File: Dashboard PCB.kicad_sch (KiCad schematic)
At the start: 40 parts

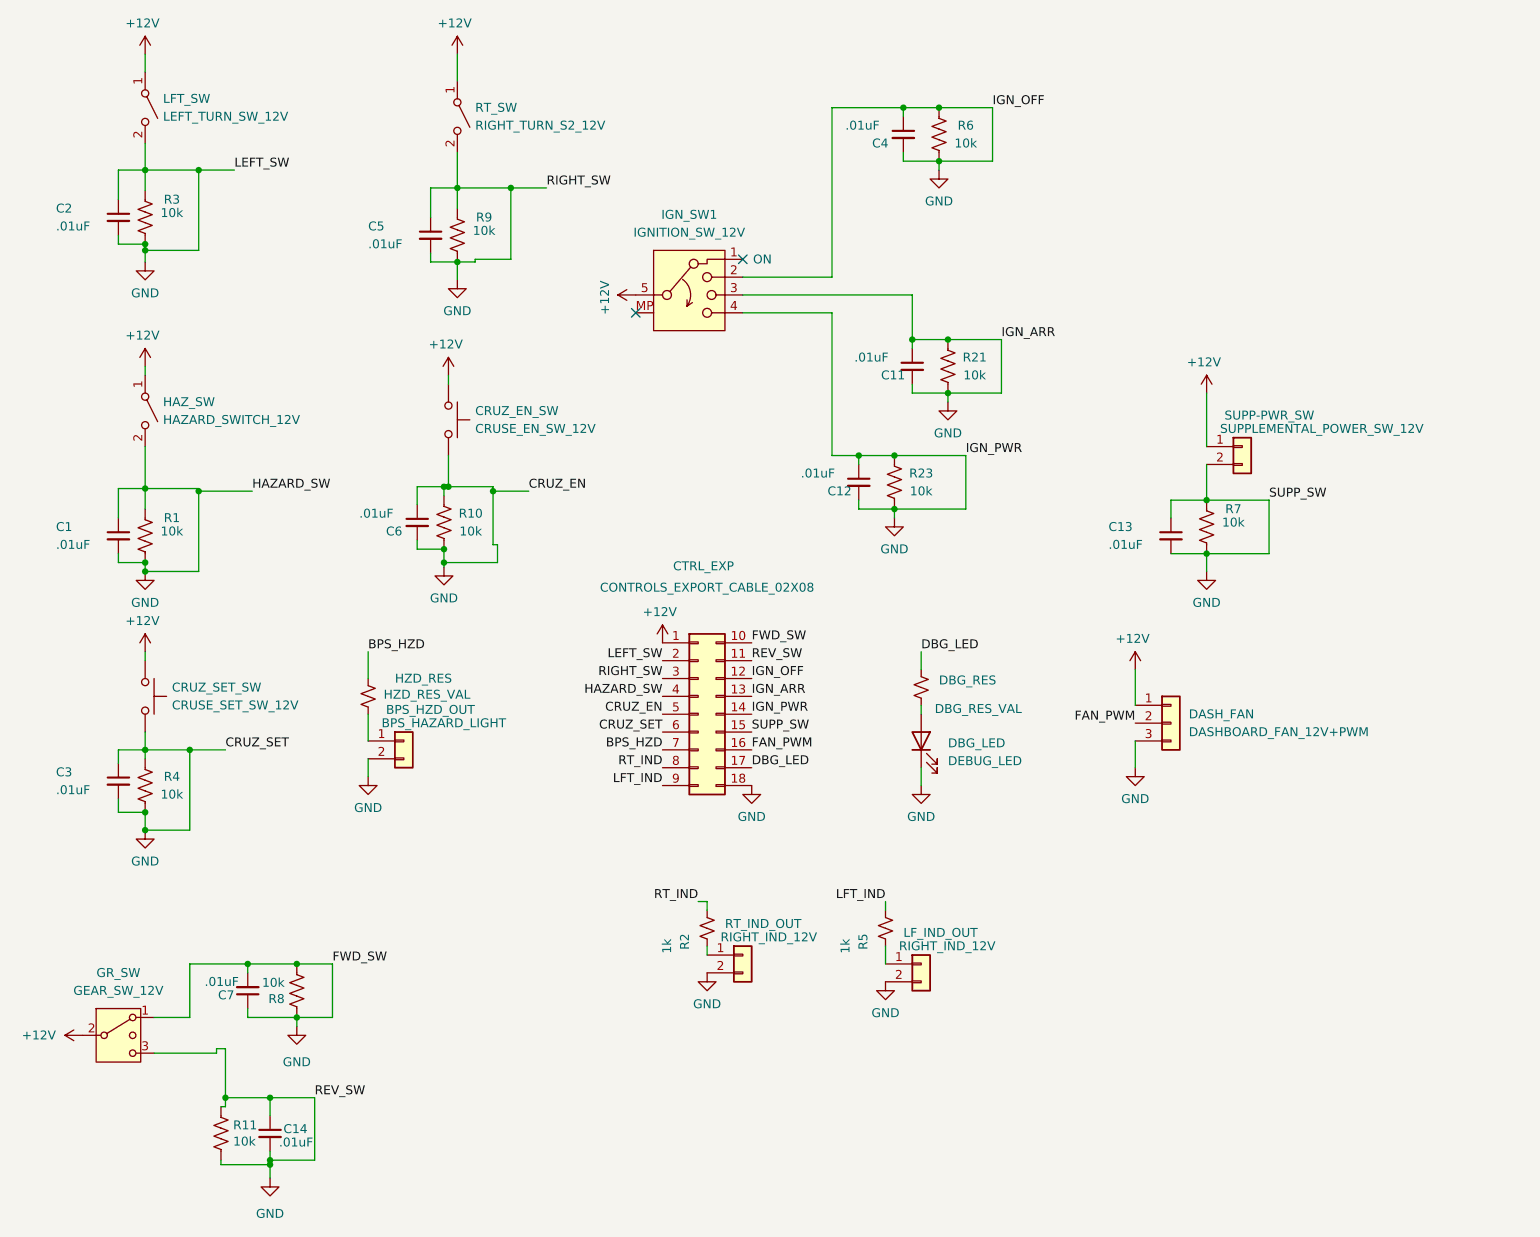
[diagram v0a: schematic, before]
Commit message: Major redisign
Added a lot of stuff and redesigned a lot of stuff
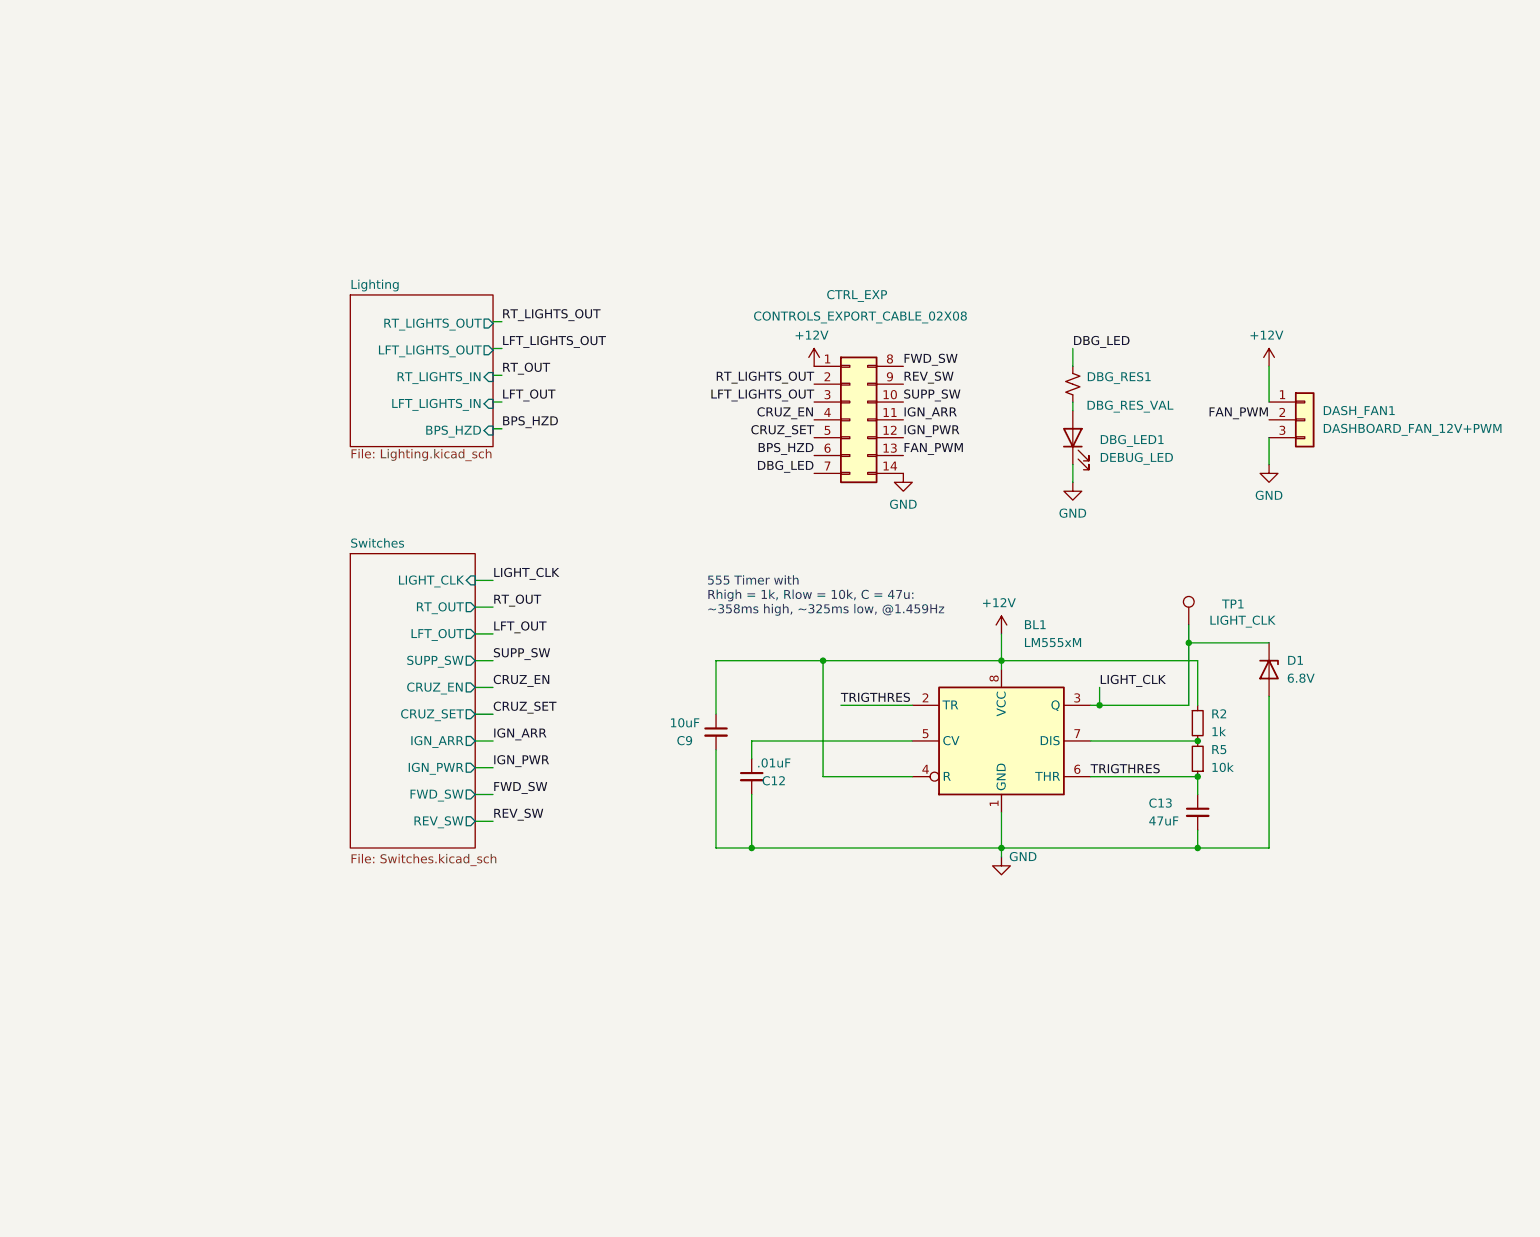
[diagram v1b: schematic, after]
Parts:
- removed BPS_HZD_OUT: BPS_HAZARD_LIGHT, Connector_Molex:Molex_Micro-Fit_3.0_43650-0215_1x02_P3.00mm_Vertical, symbol Connector_Generic:Conn_01x02
- removed C1, C11, C14, C2, C3, C4, C5, C6, C7: .01uF, Capacitor_SMD:C_0805_2012Metric, symbol Device:C_Small
- removed CRUZ_EN_SW: CRUSE_EN_SW_12V, symbol Switch:SW_Push
- removed CRUZ_SET_SW: CRUSE_SET_SW_12V, symbol Switch:SW_Push
- removed DASH_FAN: DASHBOARD_FAN_12V+PWM, symbol Connector_Generic:Conn_01x03
- removed DBG_LED: DEBUG_LED, symbol Device:LED
- removed DBG_RES: DBG_RES_VAL, Resistor_SMD:R_0805_2012Metric, symbol Device:R_Small_US
- removed GR_SW: GEAR_SW_12V, symbol Switch:SW_SPDT_MSM
- removed HAZ_SW: HAZARD_SWITCH_12V, symbol Switch:SW_SPST
- removed HZD_RES: HZD_RES_VAL, Resistor_SMD:R_0805_2012Metric, symbol Device:R_Small_US
- removed IGN_SW1: IGNITION_SW_12V, symbol Switch:SW_Rotary_1x4_MP
- removed LFT_SW: LEFT_TURN_SW_12V, symbol Switch:SW_SPST
- removed LF_IND_OUT, RT_IND_OUT: RIGHT_IND_12V, Connector_Molex:Molex_Micro-Fit_3.0_43650-0215_1x02_P3.00mm_Vertical, symbol Connector_Generic:Conn_01x02
- removed R1, R10, R11, R21, R23, R3, R4, R6, R7, R8, R9: 10k, Resistor_SMD:R_0805_2012Metric, symbol Device:R_US
- removed R2, R5: 1k, Resistor_SMD:R_0805_2012Metric, symbol Device:R_Small_US
- removed RT_SW: RIGHT_TURN_S2_12V, symbol Switch:SW_SPST
- removed SUPP-PWR_SW: SUPPLEMENTAL_POWER_SW_12V, Connector_Molex:Molex_Micro-Fit_3.0_43650-0215_1x02_P3.00mm_Vertical, symbol Connector_Generic:Conn_01x02
- added BL1: LM555xM, Package_SO:SOIC-8_3.9x4.9mm_P1.27mm, symbol Timer:LM555xM
- added C9: 10uF, Capacitor_SMD:C_0805_2012Metric, symbol Device:C_Small
- added D1: 6.8V, Diode_SMD:D_0805_2012Metric, symbol Device:D_Zener
- added DASH_FAN1: DASHBOARD_FAN_12V+PWM, symbol Connector_Generic:Conn_01x03
- added DBG_LED1: DEBUG_LED, symbol Device:LED
- added DBG_RES1: DBG_RES_VAL, Resistor_SMD:R_0805_2012Metric, symbol Device:R_Small_US
- added R2: 1k, Resistor_SMD:R_0805_2012Metric, symbol Device:R_Small
- added R5: 10k, Resistor_SMD:R_0805_2012Metric, symbol Device:R_Small
- added TP1: LIGHT_CLK, TestPoint:TestPoint_Pad_1.5x1.5mm, symbol Connector:TestPoint
- C13: value .01uF -> 47uF; P/N C0805C103J5RACTU -> C2012X5R0J476M125AC
- CTRL_EXP: symbol Connector_Generic:Conn_02x09_Top_Bottom -> Connector_Generic:Conn_02x07_Top_Bottom
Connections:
- net +12V: now also BL1.4 (R), BL1.8 (VCC), C9.1, DASH_FAN1.1 (Pin_1), R2.1
- net BPS_HZD: now also CTRL_EXP.6 (Pin_6); no longer CTRL_EXP.7 (Pin_7)
- net DBG_LED: now also CTRL_EXP.7 (Pin_7), DBG_RES1.1; no longer CTRL_EXP.17 (Pin_17)
- net FAN_PWM: now also CTRL_EXP.13 (Pin_13), DASH_FAN1.2 (Pin_2); no longer CTRL_EXP.16 (Pin_16)
- net GND: now also BL1.1 (GND), C9.2, D1.2 (A), DASH_FAN1.3 (Pin_3), DBG_LED1.1 (K); no longer C12.1, C13.1, CTRL_EXP.10 (Pin_10), CTRL_EXP.11 (Pin_11), CTRL_EXP.12 (Pin_12), CTRL_EXP.13 (Pin_13), CTRL_EXP.15 (Pin_15), CTRL_EXP.18 (Pin_18), CTRL_EXP.2 (Pin_2), CTRL_EXP.3 (Pin_3), CTRL_EXP.4 (Pin_4), CTRL_EXP.5 (Pin_5), CTRL_EXP.6 (Pin_6)
- net LFT_IND renamed REV_SW
- net RT_IND renamed FWD_SW
- new net: DBG_LED1.2 (A), DBG_RES1.2
- new net: BL1.7 (DIS), R2.2, R5.2
- new net: BL1.5 (CV), C12.1
- new net CRUZ_EN: CTRL_EXP.4 (Pin_4)
- new net CRUZ_SET: CTRL_EXP.5 (Pin_5)
- new net IGN_ARR: CTRL_EXP.11 (Pin_11)
- new net IGN_PWR: CTRL_EXP.12 (Pin_12)
- new net LFT_LIGHTS_OUT: CTRL_EXP.3 (Pin_3)
- new net LIGHT_CLK: BL1.3 (Q), D1.1 (K), TP1.1
- new net RT_LIGHTS_OUT: CTRL_EXP.2 (Pin_2)
- new net SUPP_SW: CTRL_EXP.10 (Pin_10)
- new net TRIGTHRES: BL1.2 (TR), BL1.6 (THR), C13.1, R5.1
- no-connect marks 2 -> 0
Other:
- added sheet Lighting (Lighting.kicad_sch)
- added sheet Switches (Switches.kicad_sch)
- note added: "555 Timer with Rhigh = 1k, Rlow = 10k, C = 47u: ~358ms high, ~325ms low, @1.459Hz"
- note removed: "ON"
